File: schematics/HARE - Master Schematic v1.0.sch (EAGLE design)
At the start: 93 parts, among them IC1 NE5532N, IC2 NE5532N, IC3 FT232RL, IC4 NE5532N, IC5 7805DT, IC6 AT25P, J1 9V, J2 STEREOSW, J3 STEREOSW, Q1 16 MHz, SW1 3PDT, SW2 Reset Button, U1 ATMEGA328P-PU, U2 MCP4921-E/P, X2 USB-B-H

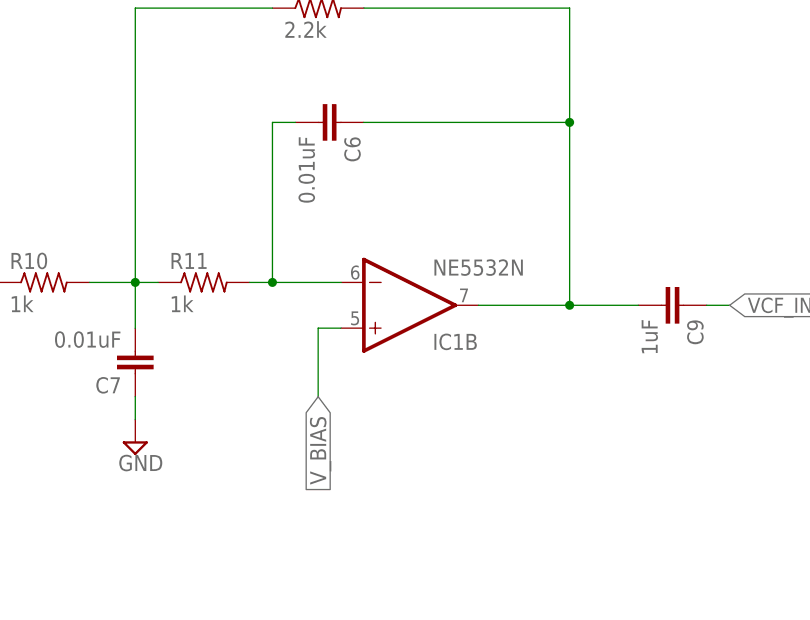
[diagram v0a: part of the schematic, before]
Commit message: Updated master schematic
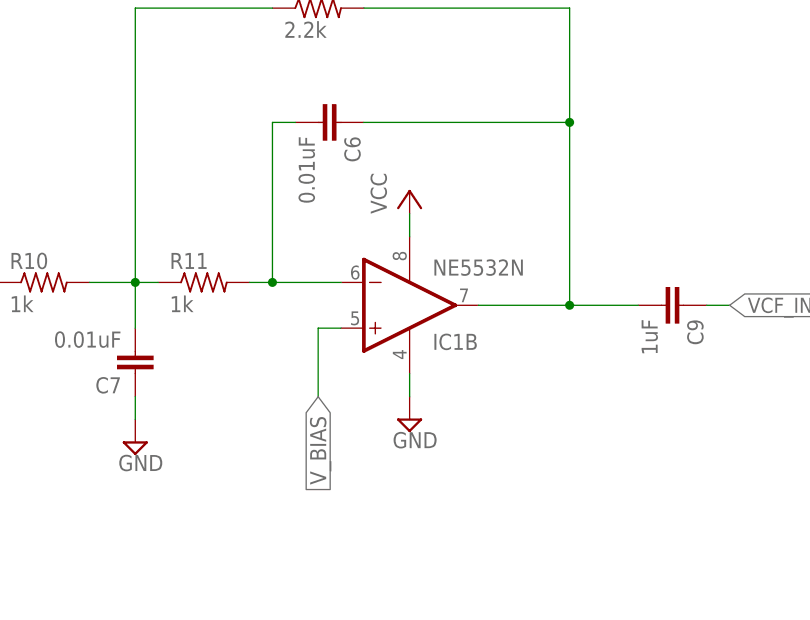
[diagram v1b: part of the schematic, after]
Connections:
- net GND: now also IC1P.V-
- net VCC: now also IC1P.V+
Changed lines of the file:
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@@
 <part name="SUPPLY9" library="supply2" deviceset="GND" device=""/>
 <part name="C5" library="resistor" deviceset="C-EU" device="C0805K" value="1uF"/>
+<part name="SUPPLY10" library="supply2" deviceset="GND" device=""/>
+<part name="P+5" library="supply1" deviceset="VCC" device=""/>
 </parts>
 <sheets>
@@
 <instance part="SUPPLY9" gate="GND" x="203.2" y="208.28"/>
 <instance part="C5" gate="G$1" x="139.7" y="215.9" rot="R90"/>
+<instance part="IC1" gate="P" x="309.88" y="233.68"/>
+<instance part="SUPPLY10" gate="GND" x="309.88" y="220.98"/>
+<instance part="P+5" gate="VCC" x="309.88" y="246.38"/>
 </instances>
 <busses>
@@
 <pinref part="P+8" gate="VCC" pin="VCC"/>
 <wire x1="154.94" y1="271.78" x2="154.94" y2="274.32" width="0.1524" layer="91"/>
+</segment>
+<segment>
+<pinref part="IC1" gate="P" pin="V+"/>
+<pinref part="P+5" gate="VCC" pin="VCC"/>
+<wire x1="309.88" y1="241.3" x2="309.88" y2="243.84" width="0.1524" layer="91"/>
 </segment>
 </net>
@@
 <junction x="203.2" y="215.9"/>
 </segment>
+<segment>
+<pinref part="SUPPLY10" gate="GND" pin="GND"/>
+<pinref part="IC1" gate="P" pin="V-"/>
+<wire x1="309.88" y1="223.52" x2="309.88" y2="226.06" width="0.1524" layer="91"/>
+</segment>
 </net>
 <net name="INPUT" class="0">
@@
 </sheet>
 </sheets>
-<errors>
-</errors>
 </schematic>
 </drawing>
